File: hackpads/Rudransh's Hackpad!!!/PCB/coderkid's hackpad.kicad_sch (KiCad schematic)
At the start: 31 parts, among them U2 SEEED-XIAO

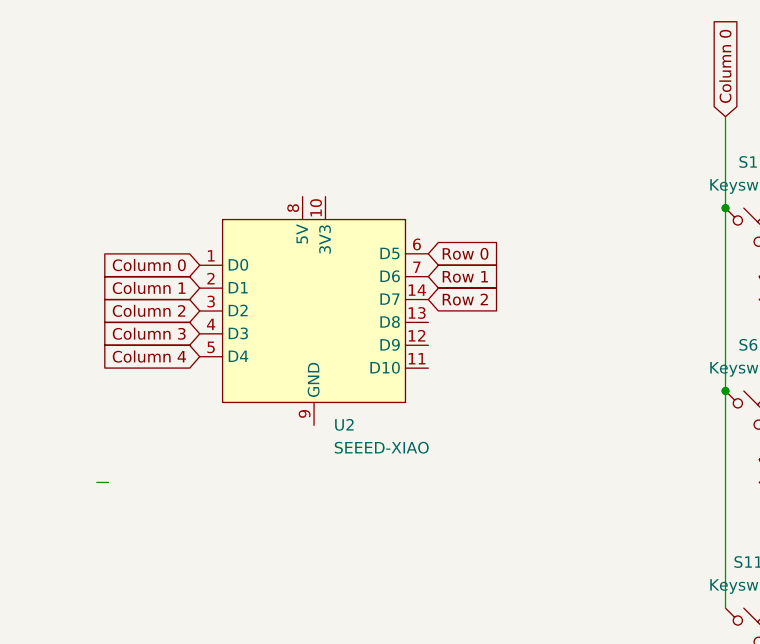
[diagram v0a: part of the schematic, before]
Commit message: UPDATED PCB files
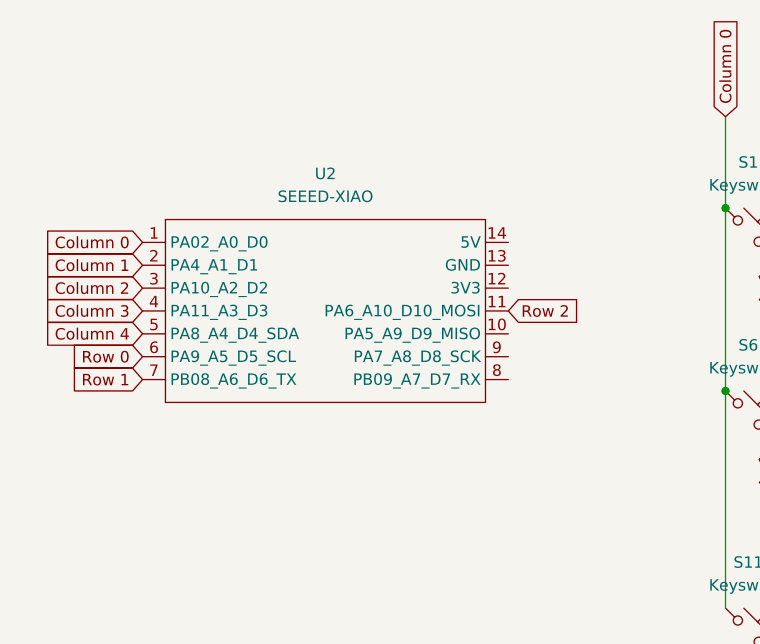
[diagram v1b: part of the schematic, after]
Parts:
- U2: footprint ScottoKeebs_MCU:Seeed_XIAO_RP2040 -> footprints:XIAO-Generic-Hybrid-14P-2.54-21X17.8MM; symbol SEEED-XIAO:SEEED-XIAO -> XIAO_RP2040:MOUDLE-SEEEDUINO-XIAO
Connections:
- net Row 2: now also U2.11 (PA6_A10_D10_MOSI); no longer U2.14 (D7)
